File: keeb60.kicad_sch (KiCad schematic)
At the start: 123 parts, among them K000 Esc, K001 1, K002 2, K003 3, K004 4, K005 5, K006 6, K007 7, K008 8, K009 9, K010 0, K011 _, K012 =, K013 Backspace, K100 Tab, K101 Q, K102 W, K103 E, K104 R, K105 T, K106 Y, K107 U, K108 I, K109 O, K110 P, K111 [, K112 ], K113 Pipe, K200 Caps Lock, K201 A, K202 S, K203 D, K204 F, K205 G, K206 H, K207 J, K208 K, K209 L, K210 ;, K211 ,, K213 Enter, K300 Shift, K302 Z, K303 X, K304 C, K305 V, K306 B, K307 N, K308 M, K309 ,, K310 ., K311 /, K313 Shift, K400 Ctrl, K401 Option, K402 Command, K406 Space, K410 Command, K411 Option, K412 Function, K413 Ctrl, U1 ProMicro

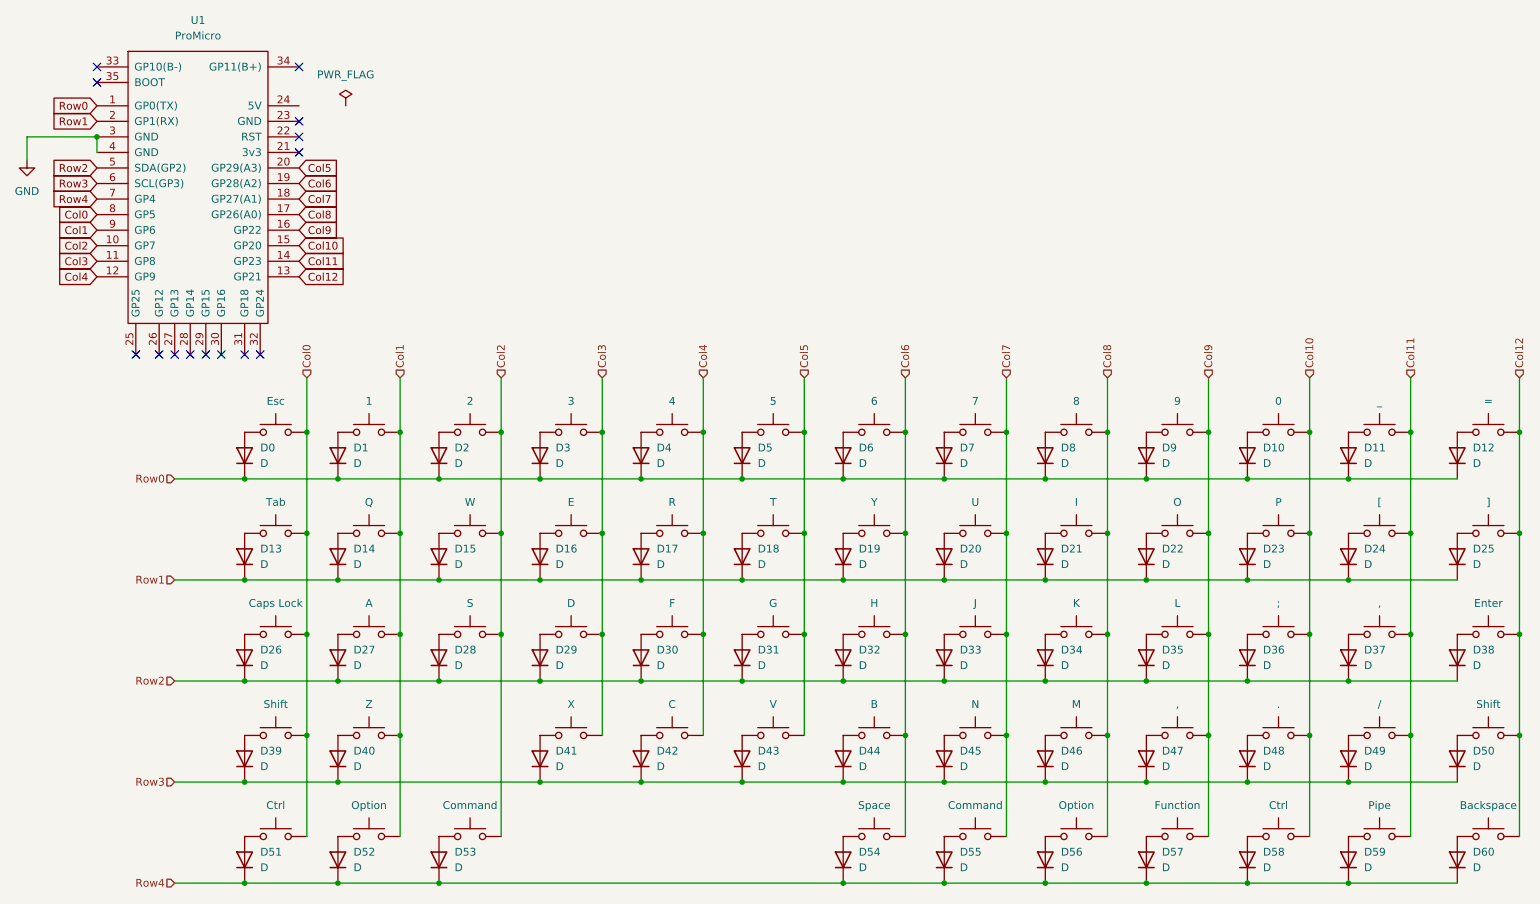
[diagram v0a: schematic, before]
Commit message: ~~magic~~
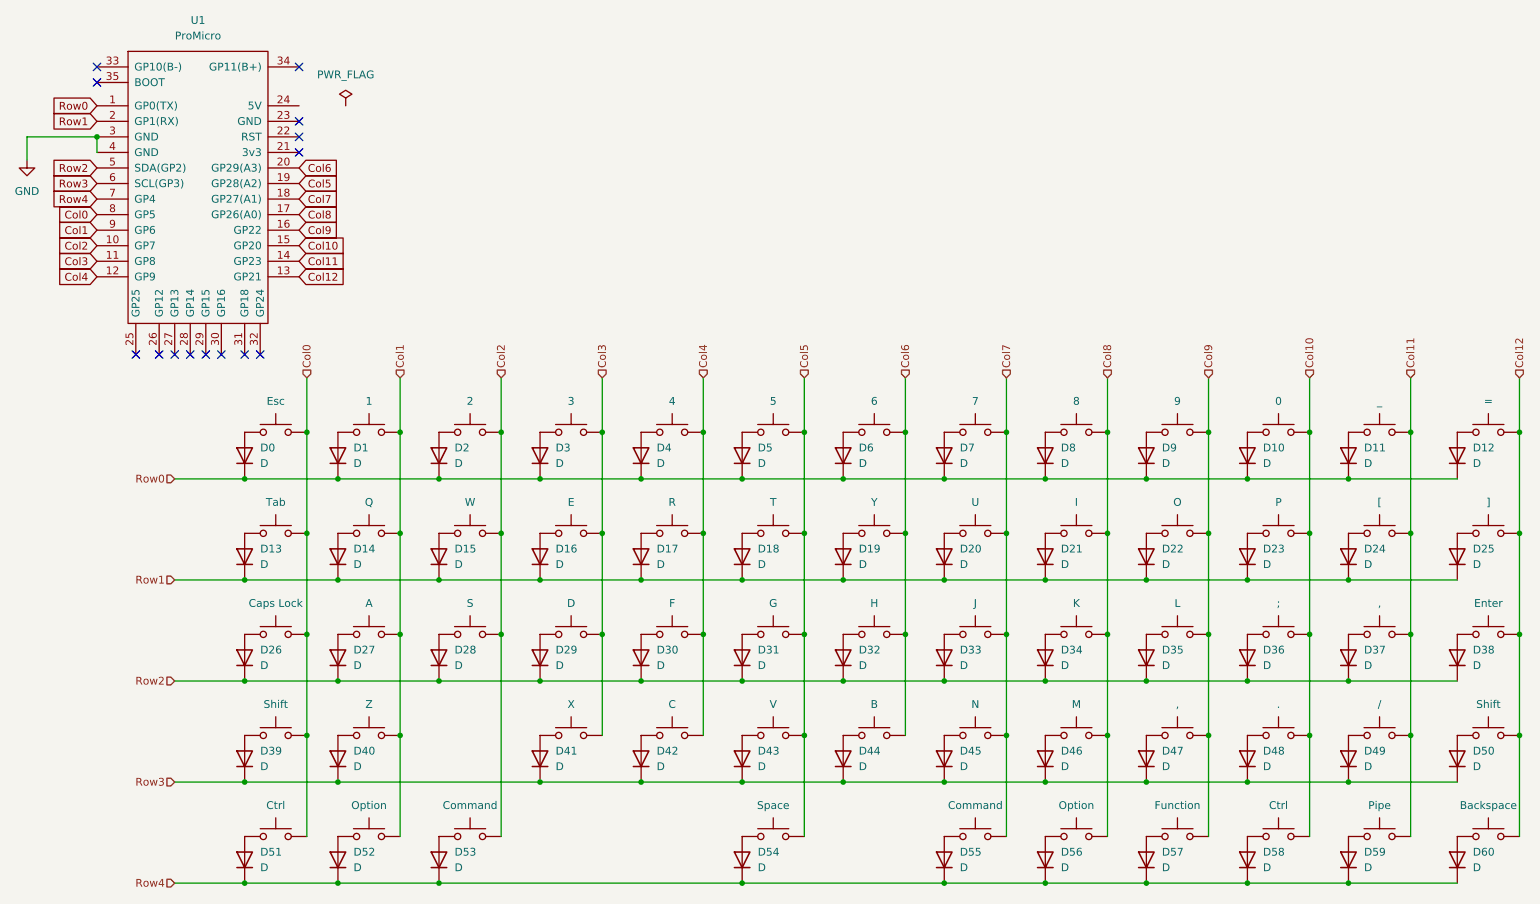
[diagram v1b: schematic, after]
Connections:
- net Col5: now also K406.2, U1.19 (GP28(A2)); no longer U1.20 (GP29(A3))
- net Col6: now also U1.20 (GP29(A3)); no longer K406.2, U1.19 (GP28(A2))
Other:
- moved on the sheet: D54
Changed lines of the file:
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@@
 	)
 	(junction
+		(at 143.51 133.35)
+		(diameter 0)
+		(color 0 0 0 0)
+	)
+	(junction
 		(at 209.55 133.35)
 		(diameter 0)
@@
 	)
 	(junction
-		(at 160.02 133.35)
-		(diameter 0)
-		(color 0 0 0 0)
-	)
-	(junction
 		(at 100.33 91.44)
 		(diameter 0)
@@
 	)
 	(junction
+		(at 133.35 157.48)
+		(diameter 0)
+		(color 0 0 0 0)
+	)
+	(junction
 		(at 226.06 116.84)
 		(diameter 0)
@@
 	)
 	(junction
-		(at 149.86 157.48)
-		(diameter 0)
-		(color 0 0 0 0)
-	)
-	(junction
 		(at 215.9 157.48)
 		(diameter 0)
@@
 	(wire
 		(pts
-			(xy 149.86 157.48) (xy 166.37 157.48)
+			(xy 83.82 157.48) (xy 133.35 157.48)
 		)
 		(stroke
@@
 	(wire
 		(pts
+			(xy 133.35 157.48) (xy 166.37 157.48)
+		)
+		(stroke
+			(width 0)
+			(type default)
+		)
+	)
+	(wire
+		(pts
 			(xy 100.33 91.44) (xy 116.84 91.44)
 		)
@@
 	(wire
 		(pts
-			(xy 83.82 157.48) (xy 149.86 157.48)
-		)
-		(stroke
-			(width 0)
-			(type default)
-		)
-	)
-	(wire
-		(pts
 			(xy 116.84 91.44) (xy 133.35 91.44)
 		)
@@
 	(wire
 		(pts
-			(xy 160.02 133.35) (xy 160.02 149.86)
-		)
-		(stroke
-			(width 0)
-			(type default)
-		)
-	)
-	(wire
-		(pts
 			(xy 166.37 107.95) (xy 182.88 107.95)
 		)
@@
 	(wire
 		(pts
+			(xy 143.51 133.35) (xy 143.51 149.86)
+		)
+		(stroke
+			(width 0)
+			(type default)
+		)
+	)
+	(wire
+		(pts
 			(xy 149.86 140.97) (xy 166.37 140.97)
 		)
@@
 		)
 	)
-	(global_label "Col6"
+	(global_label "Col5"
 		(shape input)
 		(at 60.96 43.18 0)
@@
 		)
 	)
-	(global_label "Row3"
+	(global_label "Col6"
 		(shape input)
-		(at 27.94 43.18 180)
+		(at 60.96 40.64 0)
 		(fields_autoplaced yes)
 		(effects
@@
 				(size 1.27 1.27)
 			)
-			(justify right)
+			(justify left)
 		)
 		(property "Intersheetrefs" "${INTERSHEET_REFS}"
-			(at 19.9958 43.18 0)
+			(at 68.2389 40.64 0)
 			(effects
 				(font
 					(size 1.27 1.27)
 				)
-				(justify right)
+				(justify left)
 				(hide yes)
 			)
 		)
 	)
-	(global_label "Col7"
+	(global_label "Row3"
 		(shape input)
-		(at 60.96 45.72 0)
+		(at 27.94 43.18 180)
 		(fields_autoplaced yes)
 		(effects
@@
 				(size 1.27 1.27)
 			)
-			(justify left)
+			(justify right)
 		)
 		(property "Intersheetrefs" "${INTERSHEET_REFS}"
-			(at 68.2389 45.72 0)
+			(at 19.9958 43.18 0)
 			(effects
 				(font
 					(size 1.27 1.27)
 				)
-				(justify left)
+				(justify right)
 				(hide yes)
 			)
 		)
 	)
-	(global_label "Col5"
+	(global_label "Col7"
 		(shape input)
-		(at 60.96 40.64 0)
+		(at 60.96 45.72 0)
 		(fields_autoplaced yes)
 		(effects
@@
 		)
 		(property "Intersheetrefs" "${INTERSHEET_REFS}"
-			(at 68.2389 40.64 0)
+			(at 68.2389 45.72 0)
 			(effects
 				(font
@@
 	(symbol
 		(lib_id "Switch:SW_Push")
-		(at 154.94 149.86 0)
+		(at 138.43 149.86 0)
 		(unit 1)
 		(exclude_from_sim no)
@@
 		(fields_autoplaced yes)
 		(property "Reference" "K406"
-			(at 154.94 143.51 0)
+			(at 138.43 143.51 0)
 			(effects
 				(font
@@
 		)
 		(property "Value" "Space"
-			(at 154.94 144.78 0)
+			(at 138.43 144.78 0)
 			(effects
 				(font
@@
 		)
 		(property "Footprint" "MX_Hotswap:MX-Hotswap-6.25U-ReversedStabilizers"
-			(at 154.94 144.78 0)
+			(at 138.43 144.78 0)
 			(effects
 				(font
@@
 		)
 		(property "Datasheet" "~"
-			(at 154.94 144.78 0)
+			(at 138.43 144.78 0)
 			(effects
 				(font
@@
 		)
 		(property "Description" "Push button switch, generic, two pins"
-			(at 154.94 149.86 0)
+			(at 138.43 149.86 0)
 			(effects
 				(font
@@
 	(symbol
 		(lib_id "Device:D")
-		(at 149.86 153.67 90)
+		(at 133.35 153.67 90)
 		(unit 1)
 		(exclude_from_sim no)
@@
 		(fields_autoplaced yes)
 		(property "Reference" "D54"
-			(at 152.4 152.3999 90)
+			(at 135.89 152.3999 90)
 			(effects
 				(font
@@
 		)
 		(property "Value" "D"
-			(at 152.4 154.9399 90)
+			(at 135.89 154.9399 90)
 			(effects
 				(font
@@
 		)
 		(property "Footprint" "Diode_SMD:D_SOD-123"
-			(at 149.86 153.67 0)
+			(at 133.35 153.67 0)
 			(effects
 				(font
@@
 		)
 		(property "Datasheet" "~"
-			(at 149.86 153.67 0)
+			(at 133.35 153.67 0)
 			(effects
 				(font
@@
 		)
 		(property "Description" "Diode"
-			(at 149.86 153.67 0)
+			(at 133.35 153.67 0)
 			(effects
 				(font
@@
 		)
 		(property "Sim.Device" "D"
-			(at 149.86 153.67 0)
+			(at 133.35 153.67 0)
 			(effects
 				(font
@@
 		)
 		(property "Sim.Pins" "1=K 2=A"
-			(at 149.86 153.67 0)
+			(at 133.35 153.67 0)
 			(effects
 				(font

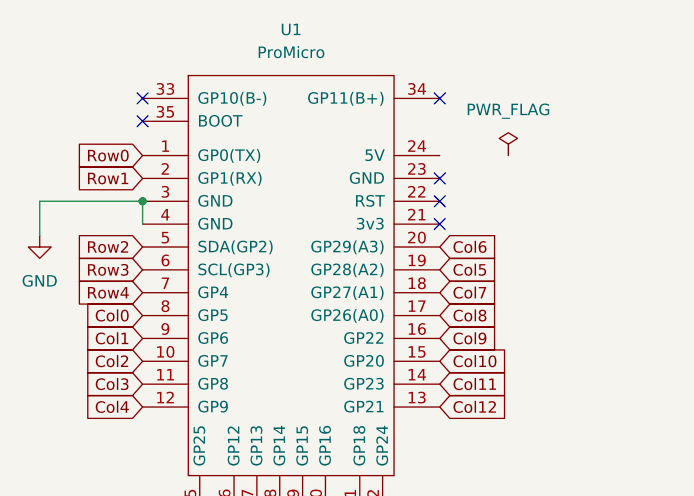
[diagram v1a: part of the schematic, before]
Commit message: Route rows
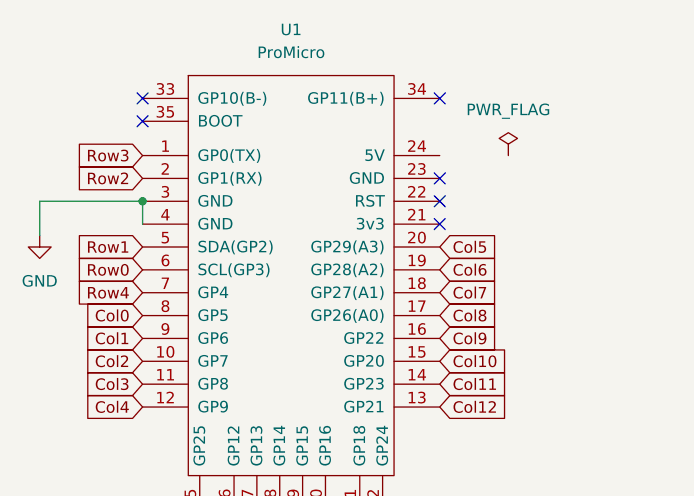
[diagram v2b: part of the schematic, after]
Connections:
- net Col5: now also U1.20 (GP29(A3)); no longer U1.19 (GP28(A2))
- net Col6: now also U1.19 (GP28(A2)); no longer U1.20 (GP29(A3))
- net Row0: now also U1.6 (SCL(GP3)); no longer U1.1 (GP0(TX))
- net Row1: now also U1.5 (SDA(GP2)); no longer U1.2 (GP1(RX))
- net Row2: now also U1.2 (GP1(RX)); no longer U1.5 (SDA(GP2))
- net Row3: now also U1.1 (GP0(TX)); no longer U1.6 (SCL(GP3))

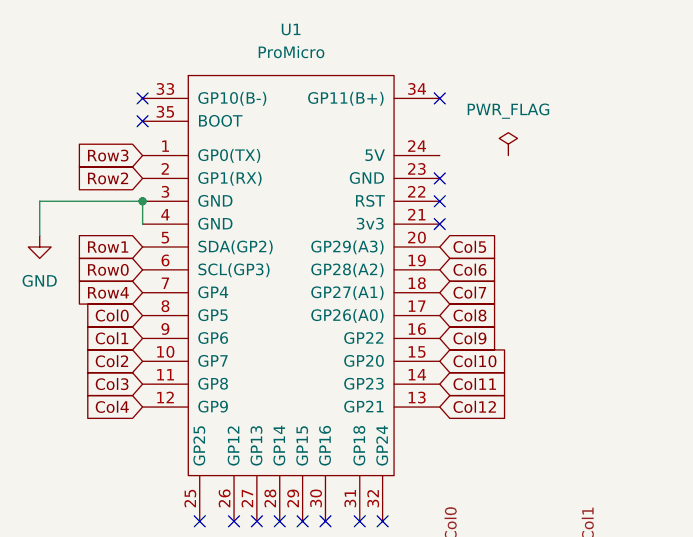
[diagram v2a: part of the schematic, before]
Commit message: Tidy
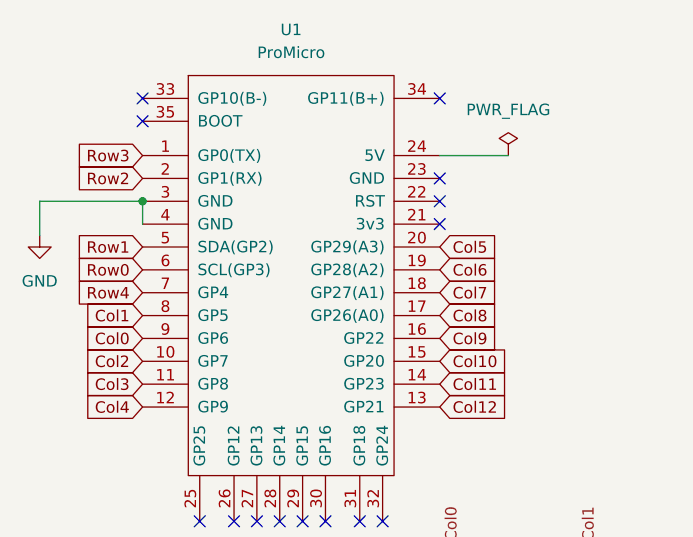
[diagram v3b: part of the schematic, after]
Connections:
- net Col0: now also U1.9 (GP6); no longer U1.8 (GP5)
- net Col1: now also U1.8 (GP5); no longer U1.9 (GP6)

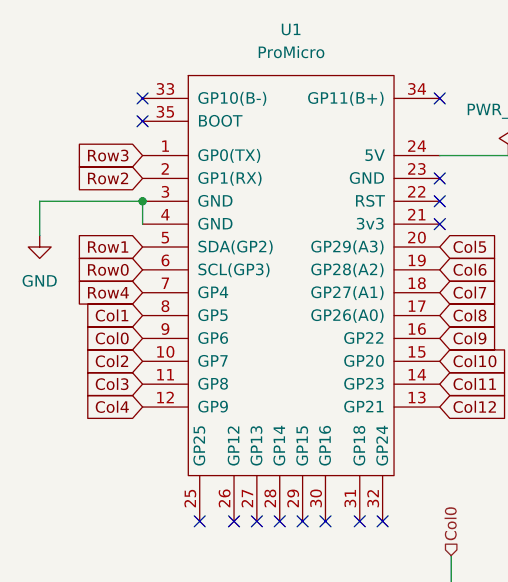
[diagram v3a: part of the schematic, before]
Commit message: Columns V2
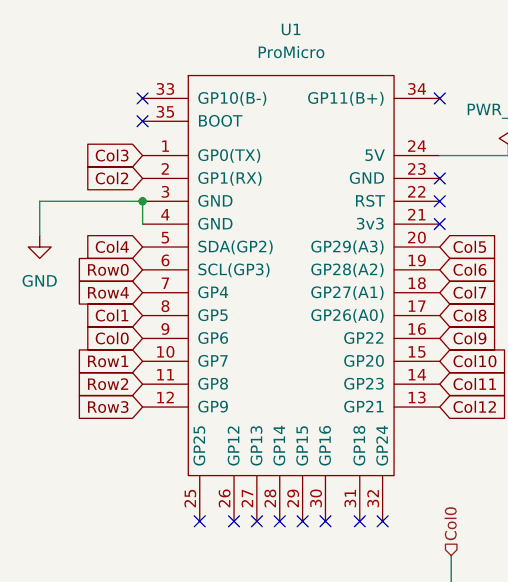
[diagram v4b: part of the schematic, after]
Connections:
- net Col2: now also U1.2 (GP1(RX)); no longer U1.10 (GP7)
- net Col3: now also U1.1 (GP0(TX)); no longer U1.11 (GP8)
- net Col4: now also U1.5 (SDA(GP2)); no longer U1.12 (GP9)
- net Row1: now also U1.10 (GP7); no longer U1.5 (SDA(GP2))
- net Row2: now also U1.11 (GP8); no longer U1.2 (GP1(RX))
- net Row3: now also U1.12 (GP9); no longer U1.1 (GP0(TX))
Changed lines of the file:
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@@
+		)
+	)
+	(global_label "Col5"
+		(shape input)
+		(at 60.96 40.64 0)
+		(fields_autoplaced yes)
+		(effects
+			(font
+				(size 1.27 1.27)
+			)
+			(justify left)
+		)
+		(property "Intersheetrefs" "${INTERSHEET_REFS}"
+			(at 68.2389 40.64 0)
+			(effects
+				(font
+					(size 1.27 1.27)
+				)
+				(justify left)
+				(hide yes)
+			)
 		)
 	)
 	(global_label "Col2"
 		(shape input)
+		(at 27.94 33.02 180)
+		(fields_autoplaced yes)
+		(effects
+			(font
+				(size 1.27 1.27)
+			)
+			(justify right)
+		)
+		(property "Intersheetrefs" "${INTERSHEET_REFS}"
+			(at 20.6611 33.02 0)
+			(effects
+				(font
+					(size 1.27 1.27)
+				)
+				(justify right)
+				(hide yes)
+			)
+		)
+	)
+	(global_label "Row3"
+		(shape input)
+		(at 27.94 58.42 180)
+		(fields_autoplaced yes)
+		(effects
+			(font
+				(size 1.27 1.27)
+			)
+			(justify right)
+		)
+		(property "Intersheetrefs" "${INTERSHEET_REFS}"
+			(at 19.9958 58.42 0)
+			(effects
+				(font
+					(size 1.27 1.27)
+				)
+				(justify right)
+				(hide yes)
+			)
+		)
+	)
+	(global_label "Col12"
+		(shape input)
+		(at 60.96 58.42 0)
+		(fields_autoplaced yes)
+		(effects
+			(font
+				(size 1.27 1.27)
+			)
+			(justify left)
+		)
+		(property "Intersheetrefs" "${INTERSHEET_REFS}"
+			(at 69.4484 58.42 0)
+			(effects
+				(font
+					(size 1.27 1.27)
+				)
+				(justify left)
+				(hide yes)
+			)
+		)
+	)
+	(global_label "Row4"
+		(shape input)
+		(at 27.94 45.72 180)
+		(fields_autoplaced yes)
+		(effects
+			(font
+				(size 1.27 1.27)
+			)
+			(justify right)
+		)
+		(property "Intersheetrefs" "${INTERSHEET_REFS}"
+			(at 19.9958 45.72 0)
+			(effects
+				(font
+					(size 1.27 1.27)
+				)
+				(justify right)
+				(hide yes)
+			)
+		)
+	)
+	(global_label "Row1"
+		(shape input)
 		(at 27.94 53.34 180)
 		(fields_autoplaced yes)
@@
 		)
 		(property "Intersheetrefs" "${INTERSHEET_REFS}"
-			(at 20.6611 53.34 0)
-			(effects
-				(font
-					(size 1.27 1.27)
-				)
-				(justify right)
-				(hide yes)
-			)
-		)
-	)
-	(global_label "Col5"
-		(shape input)
-		(at 60.96 40.64 0)
-		(fields_autoplaced yes)
-		(effects
-			(font
-				(size 1.27 1.27)
-			)
-			(justify left)
-		)
-		(property "Intersheetrefs" "${INTERSHEET_REFS}"
-			(at 68.2389 40.64 0)
-			(effects
-				(font
-					(size 1.27 1.27)
-				)
-				(justify left)
+			(at 19.9958 53.34 0)
+			(effects
+				(font
+					(size 1.27 1.27)
+				)
+				(justify right)
 				(hide yes)
 			)
@@
 	(global_label "Row2"
 		(shape input)
-		(at 27.94 33.02 180)
-		(fields_autoplaced yes)
-		(effects
-			(font
-				(size 1.27 1.27)
-			)
-			(justify right)
-		)
-		(property "Intersheetrefs" "${INTERSHEET_REFS}"
-			(at 19.9958 33.02 0)
-			(effects
-				(font
-					(size 1.27 1.27)
-				)
-				(justify right)
-				(hide yes)
-			)
-		)
-	)
-	(global_label "Col12"
-		(shape input)
-		(at 60.96 58.42 0)
-		(fields_autoplaced yes)
-		(effects
-			(font
-				(size 1.27 1.27)
-			)
-			(justify left)
-		)
-		(property "Intersheetrefs" "${INTERSHEET_REFS}"
-			(at 69.4484 58.42 0)
-			(effects
-				(font
-					(size 1.27 1.27)
-				)
-				(justify left)
-				(hide yes)
-			)
-		)
-	)
-	(global_label "Row3"
+		(at 27.94 55.88 180)
+		(fields_autoplaced yes)
+		(effects
+			(font
+				(size 1.27 1.27)
+			)
+			(justify right)
+		)
+		(property "Intersheetrefs" "${INTERSHEET_REFS}"
+			(at 19.9958 55.88 0)
+			(effects
+				(font
+					(size 1.27 1.27)
+				)
+				(justify right)
+				(hide yes)
+			)
+		)
+	)
+	(global_label "Col4"
+		(shape input)
+		(at 27.94 40.64 180)
+		(fields_autoplaced yes)
+		(effects
+			(font
+				(size 1.27 1.27)
+			)
+			(justify right)
+		)
+		(property "Intersheetrefs" "${INTERSHEET_REFS}"
+			(at 20.6611 40.64 0)
+			(effects
+				(font
+					(size 1.27 1.27)
+				)
+				(justify right)
+				(hide yes)
+			)
+		)
+	)
+	(global_label "Col3"
 		(shape input)
 		(at 27.94 30.48 180)
@@
 		)
 		(property "Intersheetrefs" "${INTERSHEET_REFS}"
-			(at 19.9958 30.48 0)
-			(effects
-				(font
-					(size 1.27 1.27)
-				)
-				(justify right)
-				(hide yes)
-			)
-		)
-	)
-	(global_label "Row4"
-		(shape input)
-		(at 27.94 45.72 180)
-		(fields_autoplaced yes)
-		(effects
-			(font
-				(size 1.27 1.27)
-			)
-			(justify right)
-		)
-		(property "Intersheetrefs" "${INTERSHEET_REFS}"
-			(at 19.9958 45.72 0)
-			(effects
-				(font
-					(size 1.27 1.27)
-				)
-				(justify right)
-				(hide yes)
-			)
-		)
-	)
-	(global_label "Col4"
-		(shape input)
-		(at 27.94 58.42 180)
-		(fields_autoplaced yes)
-		(effects
-			(font
-				(size 1.27 1.27)
-			)
-			(justify right)
-		)
-		(property "Intersheetrefs" "${INTERSHEET_REFS}"
-			(at 20.6611 58.42 0)
+			(at 20.6611 30.48 0)
 			(effects
 				(font
@@
 		)
 	)
-	(global_label "Row1"
-		(shape input)
-		(at 27.94 40.64 180)
-		(fields_autoplaced yes)
-		(effects
-			(font
-				(size 1.27 1.27)
-			)
-			(justify right)
-		)
-		(property "Intersheetrefs" "${INTERSHEET_REFS}"
-			(at 19.9958 40.64 0)
-			(effects
-				(font
-					(size 1.27 1.27)
-				)
-				(justify right)
-				(hide yes)
-			)
-		)
-	)
 	(global_label "Col10"
 		(shape input)
@@
 			(effects
 				(font
-					(size 1.27 1.27)
-				)
-				(justify right)
-				(hide yes)
-			)
-		)
-	)
-	(global_label "Col3"
-		(shape input)
-		(at 27.94 55.88 180)
-		(fields_autoplaced yes)
-		(effects
-			(font
-				(size 1.27 1.27)
-			)
-			(justify right)
-		)
-		(property "Intersheetrefs" "${INTERSHEET_REFS}"
-			(at 20.6611 55.88 0)
-			(effects
-				(font
